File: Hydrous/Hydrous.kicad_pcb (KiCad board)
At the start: 2 copper layers, 97.2 x 47.6 mm, 60 parts, among them J1 Screw_Terminal_01x02, J10 Entrada 12v, J11 Encoder, J12 PB1 (OK), J13 PB2 (RETURN), J14 Sensor de humedad, J2 Screw_Terminal_01x02, J3 Screw_Terminal_01x02, J4 Screw_Terminal_01x02, J5 Screw_Terminal_01x02, J6 Screw_Terminal_01x02, J7 Sensor de flujo, J8 Dispensador de nutrientes, J9 LCD, Q1 AO3400_C4748804, Q2 AO3400_C4748804, Q3 AO3400_C4748804, Q4 AO3400_C4748804, Q5 AO3400_C4748804, Q6 AO3400_C4748804, Q7 AO3400_C4748804, SW1 SKRPACE010, U1 L7805ABD2T-TR, U2 AMS1117-3.3_C347222, U3 ESP32-S3-WROOM-1(N16)

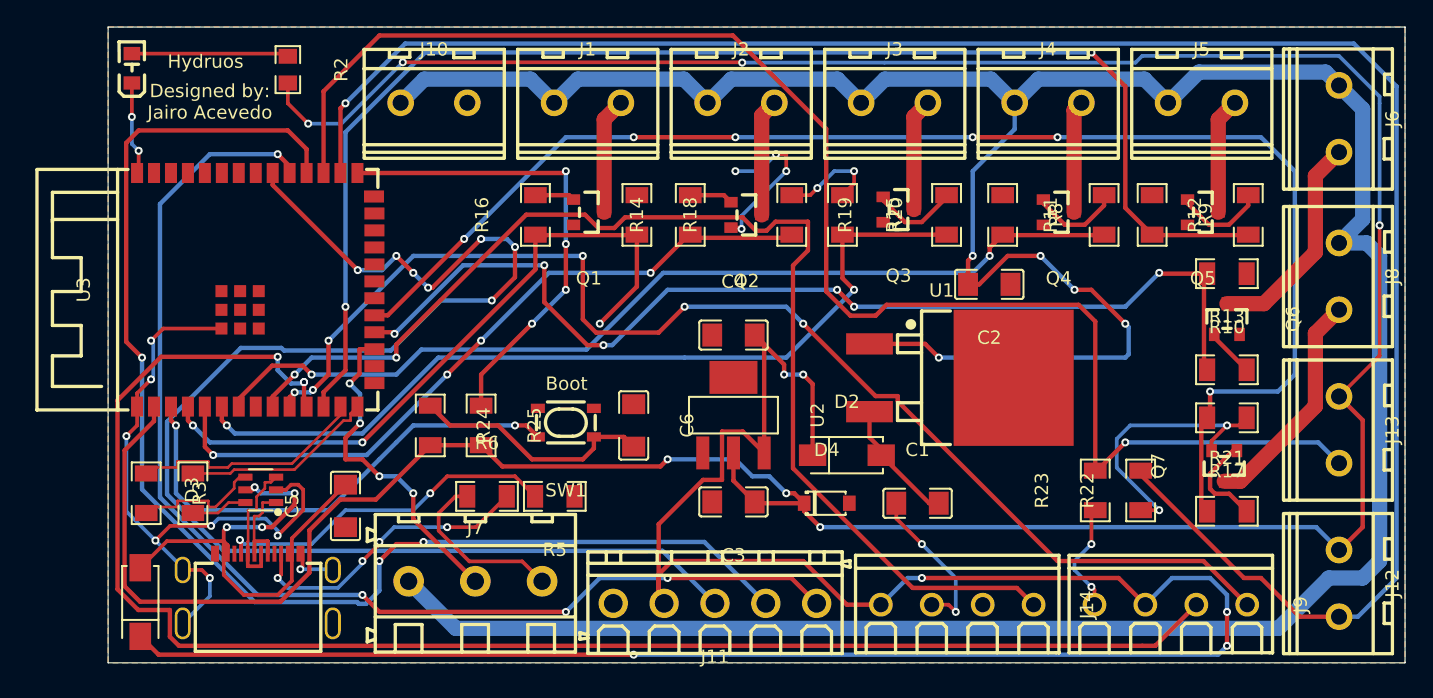
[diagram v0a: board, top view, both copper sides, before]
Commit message: Update
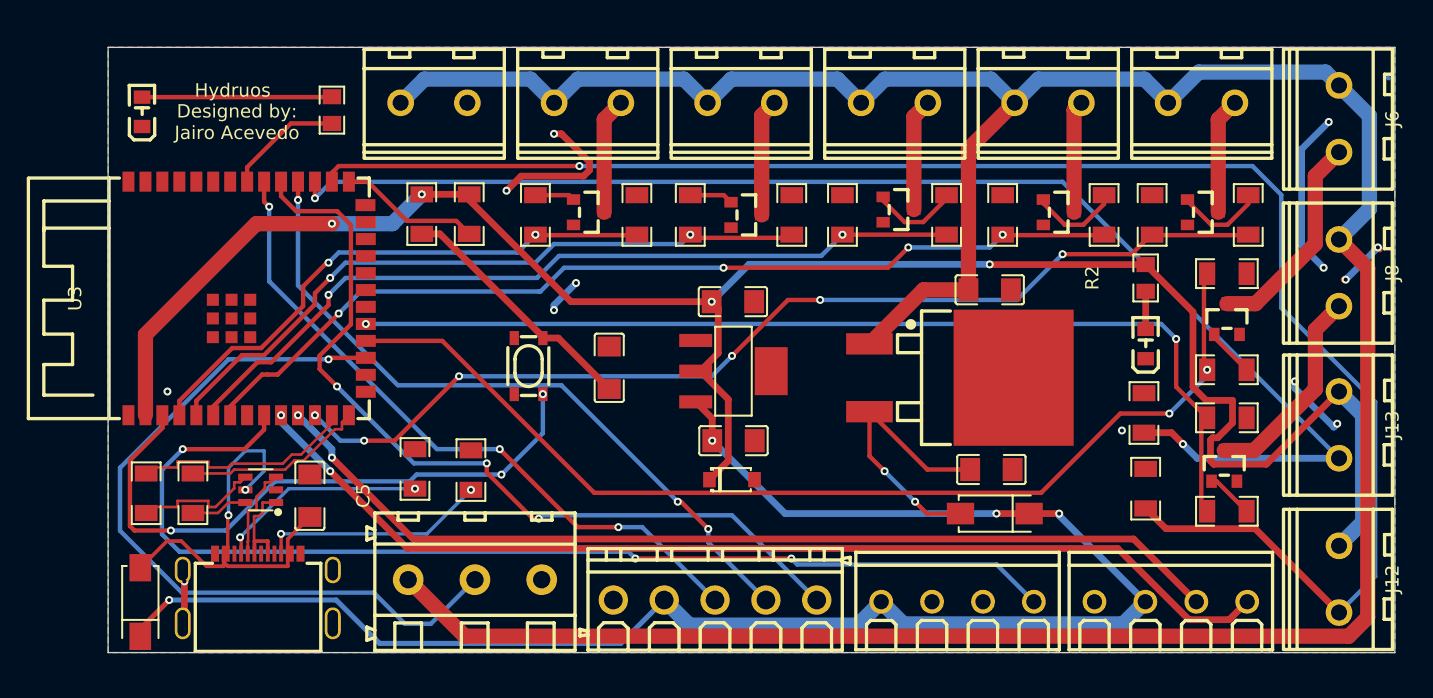
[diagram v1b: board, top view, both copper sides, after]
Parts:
- added LED4: XL-2012SURC, easyeda2kicad:LED0805-RD_RED, F.Cu at (49.5, 41.3)
- added R7: RC0805FR-0775RL, easyeda2kicad:R0805, F.Cu at (63.8, 41.1)
- moved LED3 78.7 mm to (124.7, 58.7)
- moved R2 66.1 mm to (124.7, 53.7), turned to 90 degrees
- moved R25 15.9 mm to (74.0, 48.9), turned to 90 degrees
- moved R24 15.8 mm to (70.5, 48.9), turned to 90 degrees
- moved C3 15.0 mm to (93.8, 55.5), turned to 0 degrees
- moved D2 11.9 mm to (113.4, 71.4), turned to 180 degrees
- moved R5 10.7 mm to (70.0, 68.0), turned to -90 degrees
- moved C4 7.91 mm to (93.8, 65.9), turned to 180 degrees
- moved D4 7.32 mm to (93.7, 68.8)
- moved R23 6.85 mm to (124.6, 63.8), turned to -90 degrees
- moved C1 6.08 mm to (113.2, 68.1), turned to 180 degrees
- moved SW1 5.07 mm to (78.5, 60.3), turned to -90 degrees
- moved C6 4.69 mm to (84.5, 60.5)
- moved U2 3.29 mm to (93.8, 60.7), turned to 180 degrees
- moved C5 2.77 mm to (62.1, 70.0), turned to -90 degrees
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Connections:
- net 3V3 renamed +3.3V
- U3 pad 33: unconnected-(U3-IO40-Pad33) -> LED
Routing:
- net GND: track 134.1 -> 35.4 mm, vias 23 -> 11
- net +3.3V: track 248.7 -> 150.4 mm, vias 7 -> 4
- net Switch: track 107.7 -> 50.9 mm, vias 7 -> 3
- net VCC: track 175.6 -> 123.3 mm, vias 6 -> 4
- net Out a: track 98.1 -> 53.2 mm
- net Out 08 (SCL): track 117.9 -> 73.5 mm, vias 3 -> 2
- net Flujo: track 25.1 -> 57.4 mm, vias 4 -> 1
- net Out 07: track 107.1 -> 75.4 mm, vias 6 -> 2
- net VCCQ: track 247.0 -> 220.4 mm, vias 5 -> 0
- net Net-(U3-IO0): track 35.9 -> 10.6 mm, vias 4 -> 0
- net Out b: track 88.7 -> 64.0 mm, vias 4 -> 3
- net Out 05: track 102.4 -> 77.7 mm, vias 2 -> 6
- net OUT PB1: track 149.2 -> 125.9 mm
- net Net-(LED4-A): track 0.00 -> 14.2 mm
- net Out 09 (SDA): track 93.7 -> 79.6 mm, vias 6 -> 2
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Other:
- board size 97.2 x 47.6 mm -> 96.4 x 45.3 mm
- board text removed: "Boot"
- board text removed: "ENCODER"
- board text removed: "FLUJO"
- board text removed: "HUMEDAD"
- board text removed: "LCD"
- board text removed: "Out01"
- board text removed: "Out02"
- board text removed: "Out03"
- board text removed: "Out04"
- board text removed: "Out05"
- board text removed: "Out06"
- board text removed: "Out07"
- board text removed: "PB1(OK)"
- board text removed: "PB2(BACK)"
- board text removed: "Vin(12V)"
